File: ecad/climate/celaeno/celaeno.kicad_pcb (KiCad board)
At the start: 2 copper layers, 80 x 45 mm, 72 parts, among them J10 2.10mm ID, 5.5mm OD, J11 JST PH, J12 JST PH, J4 M20-8760342, J5 47053-1000, J6 47053-1000, J7 2.10mm ID, 5.5mm OD, J8 JST PH, J9 JST PH, Q1 BSS138, Q2 BSS138, Q3 BSS138, Q4 BSS138, SW1 1825910-6, U1 LP3985IM5-3.3/NOPB, U2 AT90CAN32-16AU, U3 MCP2561-E/SN, U4 MIC4680YM, U5 CPC1966YX6, U6 EMC2302-1-AIZL-TR, Y1 16MHz

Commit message: Updates PCBs
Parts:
- J8, J9: footprint Connector_JST:JST_PH_B2B-PH-SM4-TB_1x02-1MP_P2.00mm_Vertical -> FORT:JST_PH_B2B-PH-SM4-TB_1x02-1MP_P2.00mm_Vertical
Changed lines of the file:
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@@
 			(pintype "passive")
 		)
-		(model "${KIPRJMOD}/../../lib/fort.3dshapes/47053-1000.wrl"
+		(model "${KIPRJMOD}/lib/fort.3dshapes/47053-1000.step"
 			(offset
 				(xyz 0 0 0)
@@
 			(pintype "passive")
 		)
-		(model "${KIPRJMOD}/../../lib/fort.3dshapes/47053-1000.wrl"
+		(model "${KIPRJMOD}/lib/fort.3dshapes/47053-1000.step"
 			(offset
 				(xyz 0 0 0)
@@
 		)
 	)
-	(footprint "Connector_JST:JST_PH_B2B-PH-SM4-TB_1x02-1MP_P2.00mm_Vertical"
+	(footprint "FORT:JST_PH_B2B-PH-SM4-TB_1x02-1MP_P2.00mm_Vertical"
 		(layer "F.Cu")
 		(at 181.8 93.1)
@@
 			)
 		)
-		(property "Footprint" "Connector_JST:JST_PH_B2B-PH-SM4-TB_1x02-1MP_P2.00mm_Vertical"
+		(property "Footprint" "FORT:JST_PH_B2B-PH-SM4-TB_1x02-1MP_P2.00mm_Vertical"
 			(at 0 0 0)
 			(unlocked yes)
@@
 			(roundrect_rratio 0.15625)
 		)
-		(model "${KICAD8_3DMODEL_DIR}/Connector_JST.3dshapes/JST_PH_B2B-PH-SM4-TB_1x02-1MP_P2.00mm_Vertical.wrl"
+		(model "${KIPRJMOD}/lib/fort.3dshapes/B2B-PH-SM4-TB.step"
 			(offset
-				(xyz 0 0 0)
+				(xyz 0 1.75 0)
 			)
 			(scale
@@
 			)
 			(rotate
-				(xyz 0 0 0)
+				(xyz -90 0 0)
 			)
 		)
 	)
-	(footprint "Connector_JST:JST_PH_B2B-PH-SM4-TB_1x02-1MP_P2.00mm_Vertical"
+	(footprint "FORT:JST_PH_B2B-PH-SM4-TB_1x02-1MP_P2.00mm_Vertical"
 		(layer "F.Cu")
 		(at 172.4 93.1)
@@
 			)
 		)
-		(property "Footprint" "Connector_JST:JST_PH_B2B-PH-SM4-TB_1x02-1MP_P2.00mm_Vertical"
+		(property "Footprint" "FORT:JST_PH_B2B-PH-SM4-TB_1x02-1MP_P2.00mm_Vertical"
 			(at 0 0 0)
 			(unlocked yes)
@@
 			(roundrect_rratio 0.15625)
 		)
-		(model "${KICAD8_3DMODEL_DIR}/Connector_JST.3dshapes/JST_PH_B2B-PH-SM4-TB_1x02-1MP_P2.00mm_Vertical.wrl"
+		(model "${KIPRJMOD}/lib/fort.3dshapes/B2B-PH-SM4-TB.step"
 			(offset
-				(xyz 0 0 0)
+				(xyz 0 1.75 0)
 			)
 			(scale
@@
 			)
 			(rotate
-				(xyz 0 0 0)
+				(xyz -90 0 0)
 			)
 		)

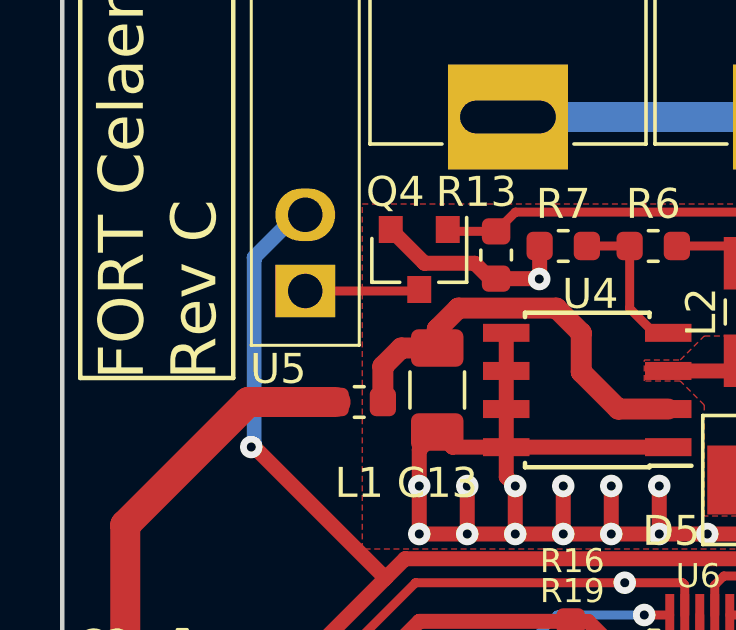
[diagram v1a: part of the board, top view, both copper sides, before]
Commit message: Flatten Arke schematics
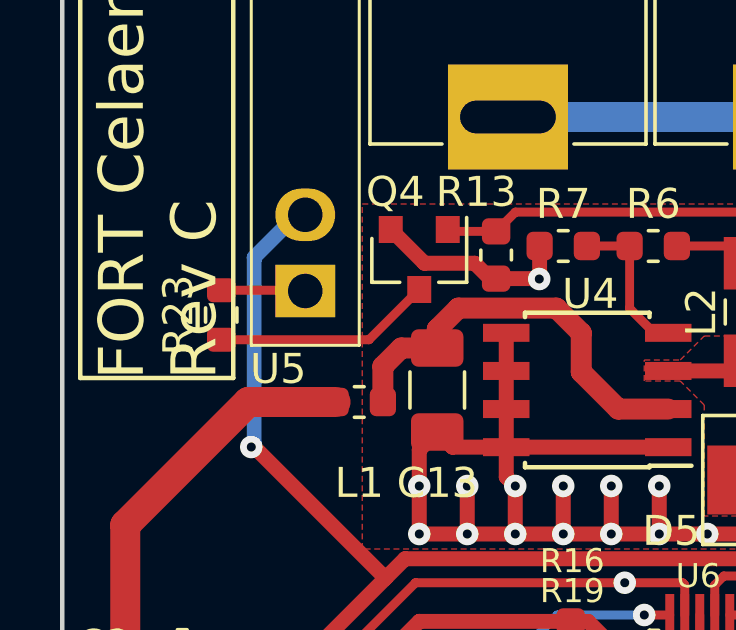
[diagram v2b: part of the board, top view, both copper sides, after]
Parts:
- added R23: 220, Resistor_SMD:R_0603_1608Metric, F.Cu at (125.3, 105.6)
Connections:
- U5 pad 1: Net-(Q4-D) -> Net-(R23-Pad2)
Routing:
- net Net-(Q4-D): track 3.82 -> 7.29 mm
- net Net-(R23-Pad2): track 0.00 -> 2.81 mm
